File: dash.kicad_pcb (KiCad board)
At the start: 2 copper layers, 48 x 70 mm, 31 parts, among them IC1 ATMEGA328-P, P1 ICSP, P2 ESP8266, P3 IN, P4 OUT, Q1 Q_NPN_CBE, Q2 Q_NPN_CBE, Q3 Q_PMOS_GDS, Q4 Q_PMOS_GDS, U1 LM317T, U2 TLC5916, Y1 16MHz

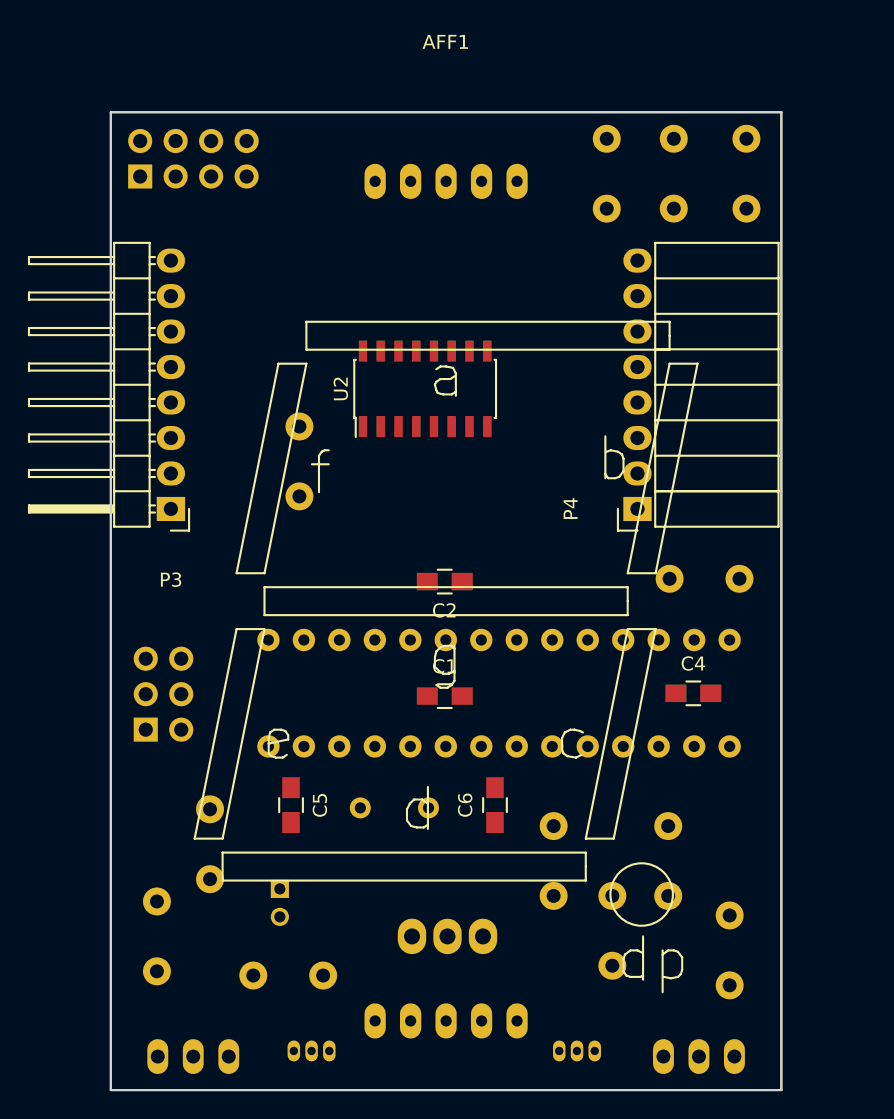
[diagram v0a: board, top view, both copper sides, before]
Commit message: Start re-routing new layout.
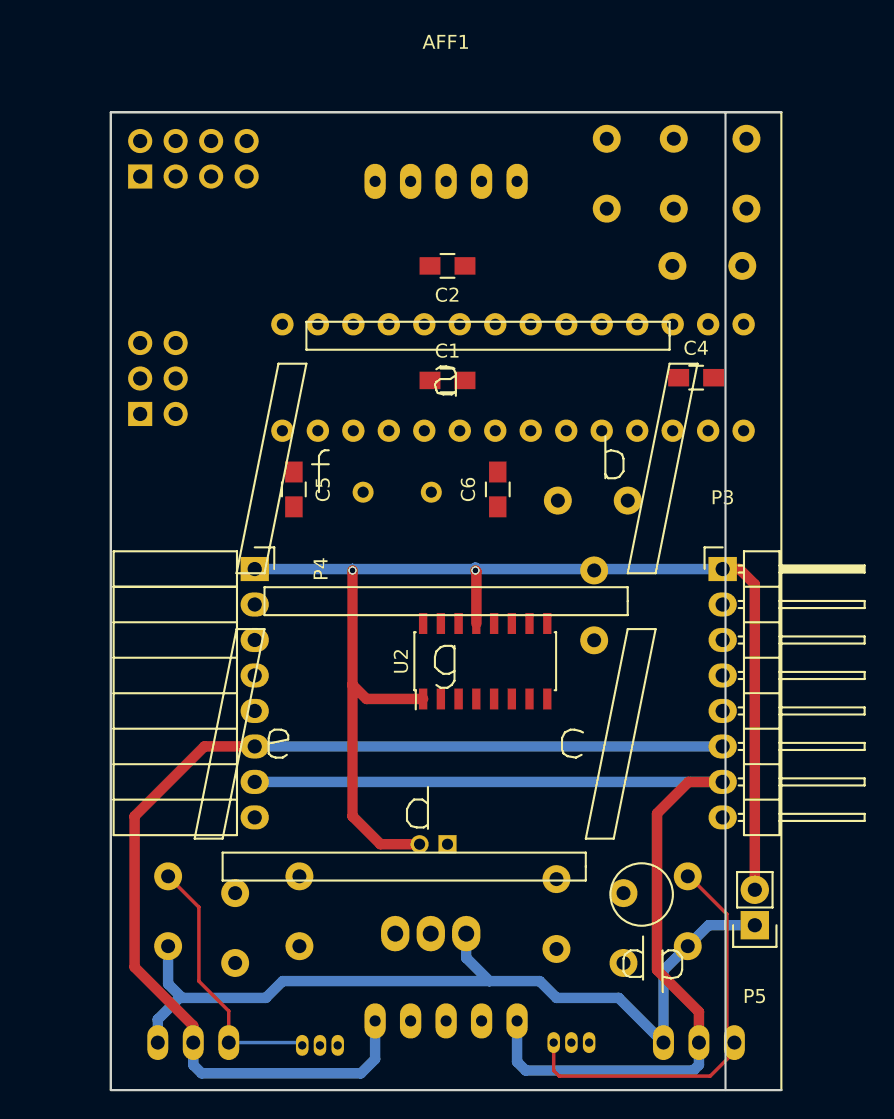
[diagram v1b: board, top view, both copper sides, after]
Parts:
- added P5: DC, Pin_Headers:Pin_Header_Straight_1x02, F.Cu at (170.6, 128.2)
- moved P3 39.7 mm to (168.3, 102.7), turned to 0 degrees
- moved P4 27.7 mm to (134.8, 102.7), turned to 270 degrees
- moved R2 26.0 mm to (159.0, 97.8), turned to 0 degrees
- moved R8 23.5 mm to (159.1, 105.3), turned to 270 degrees
- moved IC1 22.6 mm to (169.8, 92.8)
- moved P1 22.6 mm to (126.6, 91.6)
- moved C1 22.6 mm to (148.6, 89.2)
- moved C2 22.6 mm to (148.6, 81.0)
- moved C4 22.6 mm to (166.4, 89.0)
- moved C5 22.6 mm to (137.6, 97.0)
- moved C6 22.6 mm to (152.2, 97.0)
- moved Y1 22.6 mm to (145.0, 97.2)
- moved R4 22.4 mm to (167.2, 81.0)
- moved U2 20.0 mm to (151.3, 109.3)
- moved C3 12.4 mm to (148.6, 122.4), turned to 180 degrees
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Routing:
- net GND: track 0.00 -> 91.2 mm, vias 0 -> 2
- net PWR_RED: track 0.00 -> 80.1 mm
- net PWR_GREEN: track 0.00 -> 74.8 mm
- net +12V: track 0.00 -> 62.3 mm
- net Net-(Q2-Pad1): track 0.00 -> 29.8 mm
- net Net-(Q1-Pad1): track 0.00 -> 19.0 mm
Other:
- outline, holes or cut-outs redrawn
